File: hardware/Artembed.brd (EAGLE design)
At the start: 94 x 36.5 mm, 75 parts, among them J2 CORTEX_JTAG_DEBUG_MINIMUM_PTH, J3 CORTEX_JTAG_DEBUG_PTH_NS, J5 1X04_SMD_STRAIGHT_COMBO, J6 QWIIC_RIGHT_ANGLE, J7 CAMERA-HIMAX, J9 1X04_SMD_STRAIGHT_COMBO, U1 DAPLINK_KL26Z, U2 ARTEMIS_MODULESMD, U3 LIS2DH12, U4 AP2127K-1.8V, X1 16MHz, Y1 32.768kHz

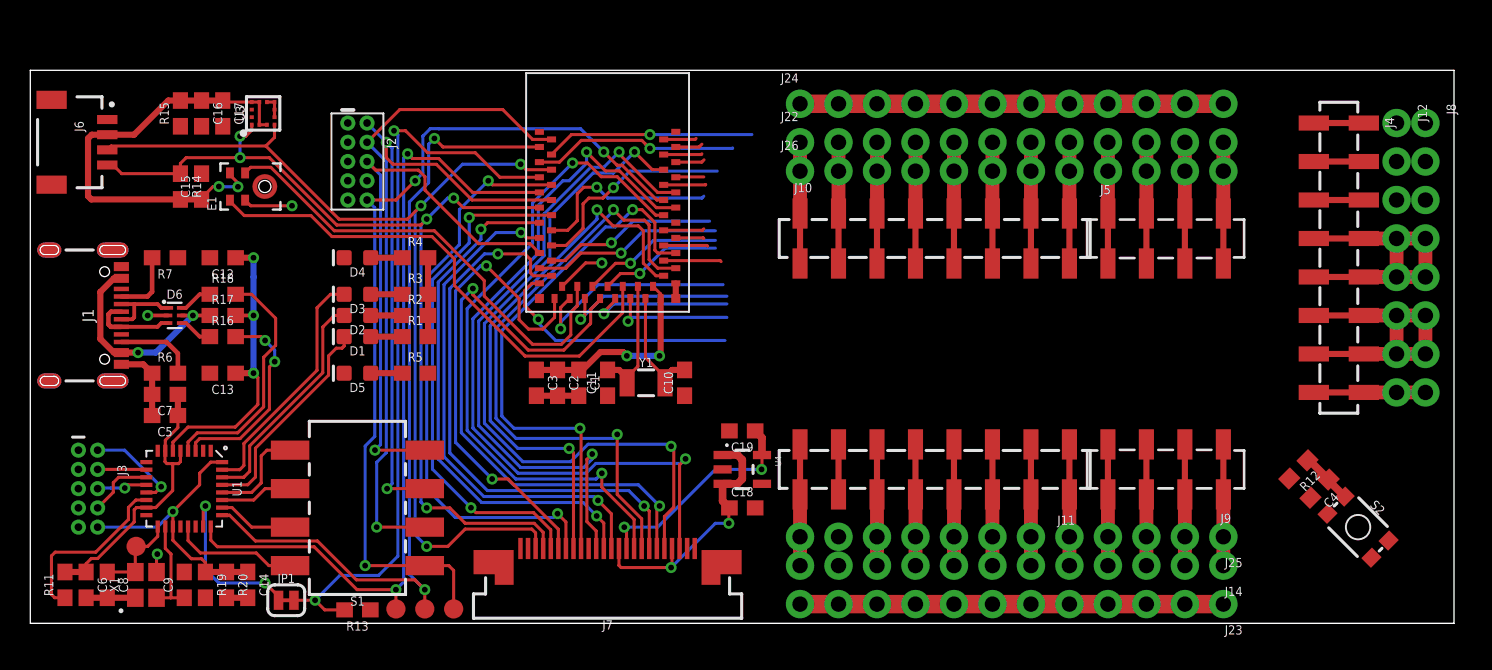
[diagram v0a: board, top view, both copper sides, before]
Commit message: routed gpio
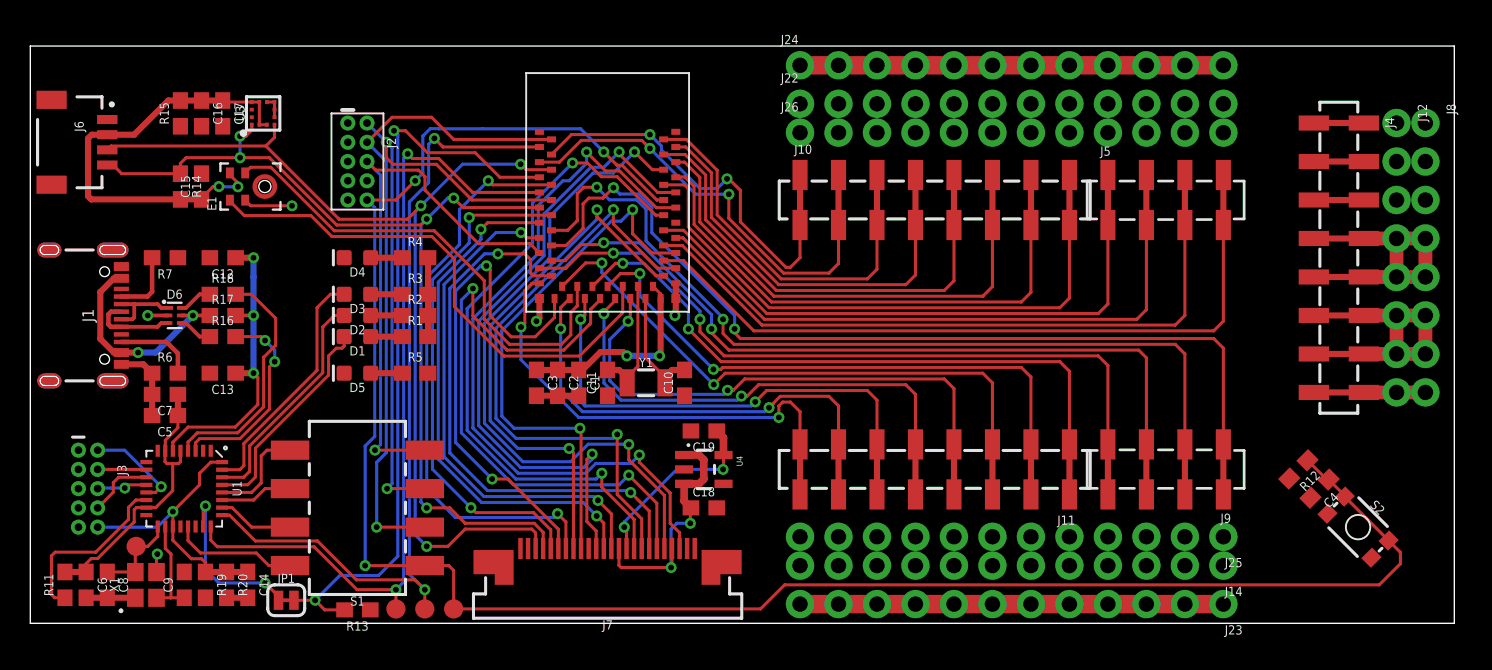
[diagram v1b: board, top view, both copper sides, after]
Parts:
- moved J10 2.54 mm to (50.8, 27.9)
- moved J5 2.54 mm to (71.1, 27.9)
- moved C18 2.54 mm to (44.5, 7.62)
- moved C19 2.54 mm to (44.5, 12.7)
- moved J22 2.54 mm to (50.8, 34.3)
- moved J24 2.54 mm to (50.8, 36.8)
- moved J26 2.54 mm to (50.8, 32.4)
- moved U4 2.54 mm to (44.5, 10.2)
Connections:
- net D13: now also J11.1, J11.1@2, J14.5, J25.5; no longer J22.12, J26.12, J5.4, J5.4-2
- net D16: now also J22.12, J26.12, J5.4, J5.4-2; no longer J22.11, J26.11, J5.3, J5.3-2
- net D23_LED: now also J14.3, J25.3, J9.3, J9.3-2; no longer J10.4, J10.4@2, J22.4, J26.4
- net D24: now also J14.1, J25.1, J9.1, J9.1-2; no longer J10.3, J10.3@2, J22.3, J26.3
- net D25: now also J11.7, J11.7@2, J14.11, J25.11; no longer J10.2, J10.2@2, J22.2, J26.2
- net D26: now also J11.6, J11.6@2, J14.10, J25.10; no longer J10.1, J10.1@2, J22.1, J26.1
- net D27: now also J14.4, J25.4, J9.4, J9.4-2; no longer J11.8, J11.8@2, J14.12, J25.12
- net D28: now also J11.8, J11.8@2, J14.12, J25.12; no longer J11.7, J11.7@2, J14.11, J25.11
- net D29: now also J11.4, J11.4@2, J14.8, J25.8; no longer J22.10, J26.10, J5.2, J5.2-2
- net D31: now also J22.11, J26.11, J5.3, J5.3-2; no longer J22.9, J26.9, J5.1, J5.1-2
- net D32: now also J11.3, J11.3@2, J14.7, J25.7; no longer J10.8, J10.8@2, J22.8, J26.8
- net D33: now also J11.2, J11.2@2, J14.6, J25.6; no longer J10.7, J10.7@2, J22.7, J26.7
- net D34: now also J11.5, J11.5@2, J14.9, J25.9; no longer J10.6, J10.6@2, J22.6, J26.6
- net D35: now also J14.2, J25.2, J9.2, J9.2-2; no longer J10.5, J10.5@2, J22.5, J26.5
- net D36: now also J10.6, J10.6@2, J22.6, J26.6; no longer J11.6, J11.6@2, J14.10, J25.10
- net D37: now also J10.4, J10.4@2, J22.4, J26.4; no longer J11.5, J11.5@2, J14.9, J25.9
- net D38: now also J10.5, J10.5@2, J22.5, J26.5; no longer J11.4, J11.4@2, J14.8, J25.8
- net D39: now also J10.1, J10.1@2, J22.1, J26.1; no longer J11.3, J11.3@2, J14.7, J25.7
- net D40: now also J10.2, J10.2@2, J22.2, J26.2; no longer J11.2, J11.2@2, J14.6, J25.6
- net D41: now also J22.10, J26.10, J5.2, J5.2-2; no longer J11.1, J11.1@2, J14.5, J25.5
- net D42: now also J10.7, J10.7@2, J22.7, J26.7; no longer J14.4, J25.4, J9.4, J9.4-2
- net D43: now also J10.8, J10.8@2, J22.8, J26.8; no longer J14.3, J25.3, J9.3, J9.3-2
- net D44: now also J10.3, J10.3@2, J22.3, J26.3; no longer J14.2, J25.2, J9.2, J9.2-2
- net D45: now also J22.9, J26.9, J5.1, J5.1-2; no longer J14.1, J25.1, J9.1, J9.1-2
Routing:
- net !TGT_RST: track 62.1 -> 131.3 mm
- net D24: track 18.6 -> 59.3 mm, vias 1 -> 2
- net D35: track 17.3 -> 56.4 mm, vias 1 -> 2
- net D16: track 8.52 -> 45.5 mm
- net D31: track 7.62 -> 42.8 mm
- net D23_LED: track 16.2 -> 49.3 mm, vias 1 -> 2
- net D41: track 6.57 -> 39.1 mm
- net D45: track 7.39 -> 37.1 mm
- net D27: track 17.3 -> 47.0 mm, vias 1 -> 2
- net D32: track 7.96 -> 37.4 mm, vias 1 -> 2
- net D43: track 7.48 -> 36.7 mm
- net D13: track 14.1 -> 40.7 mm, vias 1 -> 2
- net D42: track 6.56 -> 33.1 mm
- net D36: track 6.63 -> 30.6 mm
- net D33: track 12.9 -> 36.5 mm, vias 1 -> 2
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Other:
- board size 94 x 36.5 mm -> 94 x 38.1 mm
